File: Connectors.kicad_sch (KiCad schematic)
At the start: 44 parts, among them J1 SM05B-GHS-TB, J10 Header1x3Pin, J15 SM07B-GHS-TB, J16 SM02B-GHS-TB, J18 USB_C_Receptacle, J4 SM05B-GHS-TB, J6 SM05B-GHS-TB, J6 SM07B-GHS-TB, J8 Header1x3Pin, U10 USBLC6-4SC6, U11 USBLC6-4SC6, U12 USBLC6-4SC6, U13 USBLC6-4SC6, U14 USBLC6-4SC6, U15 USBLC6-4SC6, U16 USBLC6-4SC6, U17 USBLC6-4SC6, U18 USBLC6-4SC6, U19 USBLC6-4SC6, U20 USBLC6-4SC6, U8 USBLC6-4SC6, U9 USBLC6-4SC6

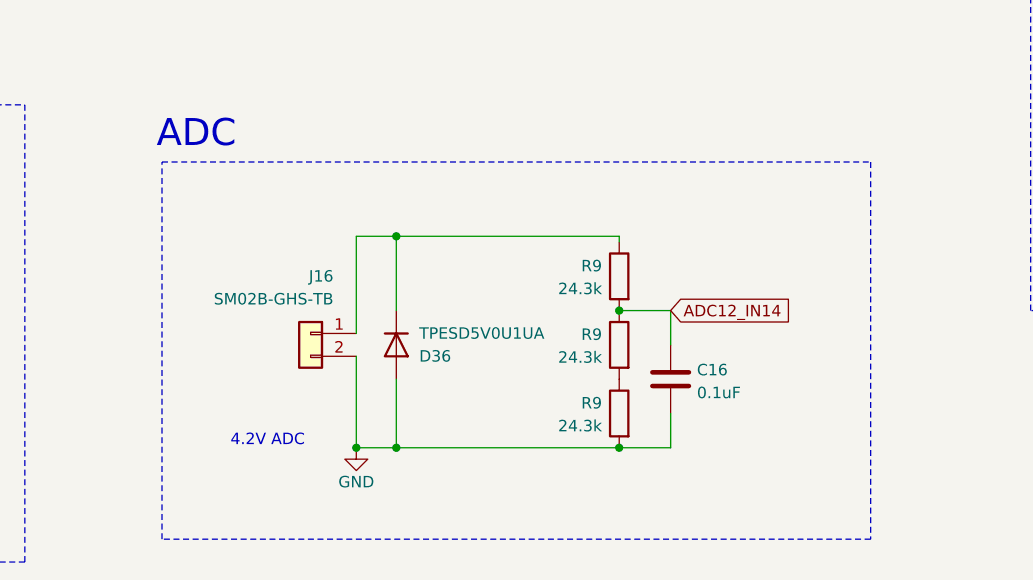
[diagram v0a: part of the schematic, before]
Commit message: Add files via upload
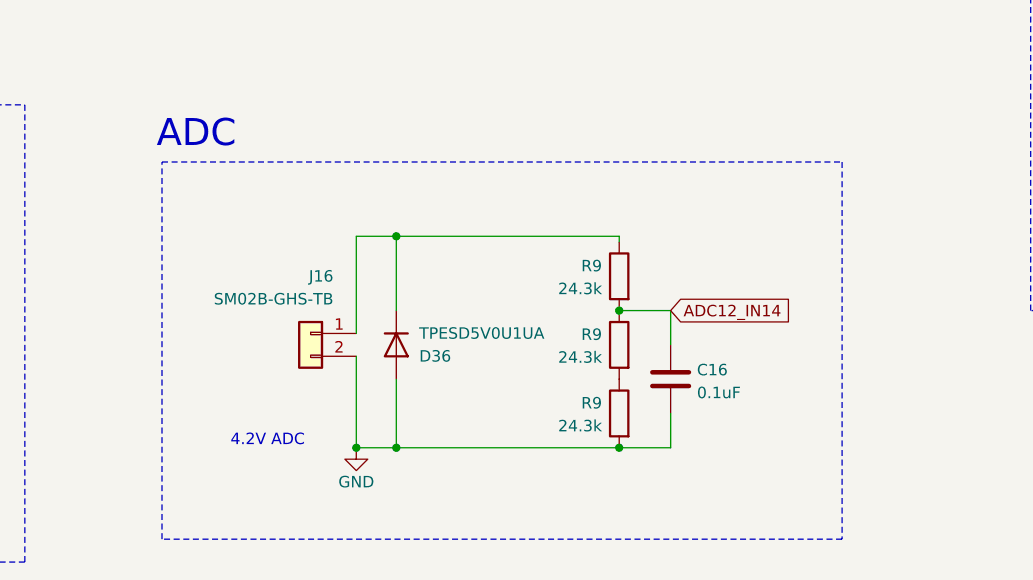
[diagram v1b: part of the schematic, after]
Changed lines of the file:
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@@
     (fill (type none))
   )
-  (rectangle (start 145.415 229.87) (end 224.155 271.78)
+  (rectangle (start 145.415 229.87) (end 220.98 271.78)
     (stroke (width 0) (type dash))
     (fill (type none))
